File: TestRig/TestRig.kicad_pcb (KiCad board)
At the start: 2 copper layers, 62 x 48 mm, 17 parts, among them J1 USB_B_Micro, J2 AVR-ISP-6

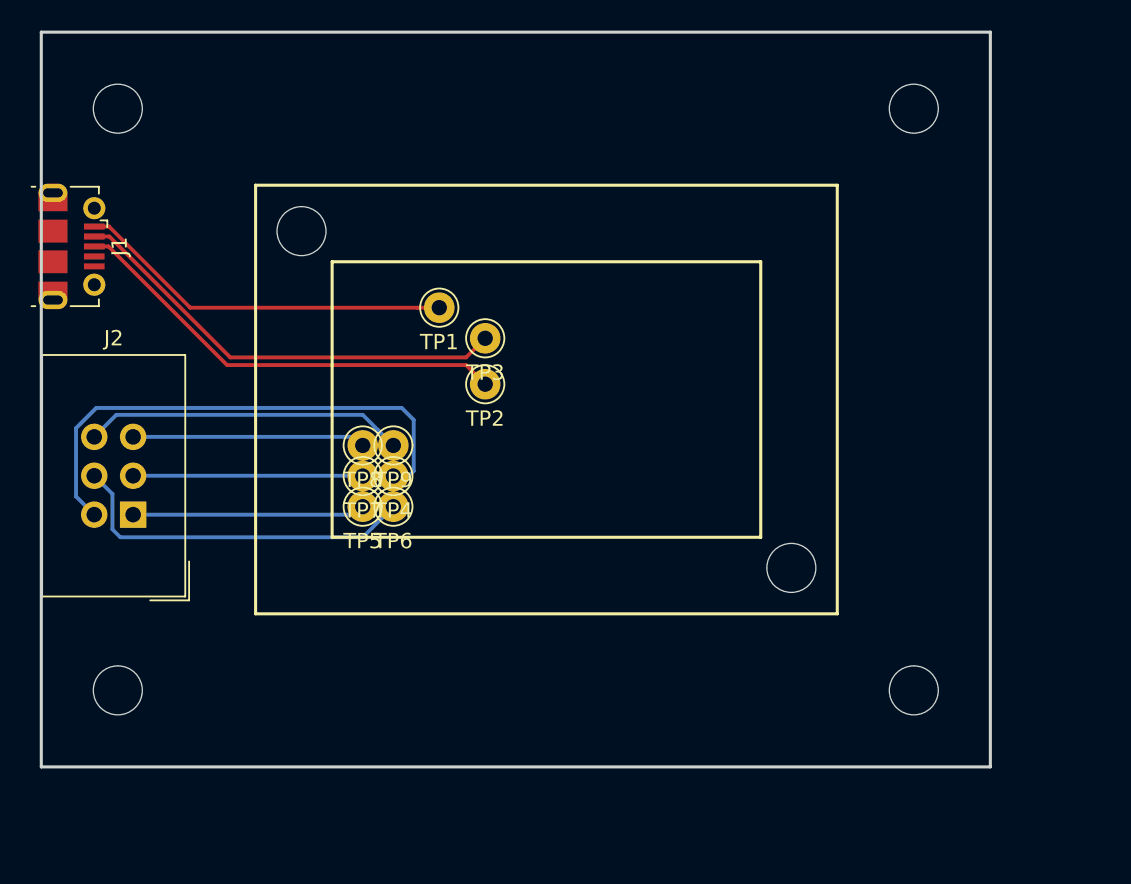
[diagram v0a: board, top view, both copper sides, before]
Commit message: Should...
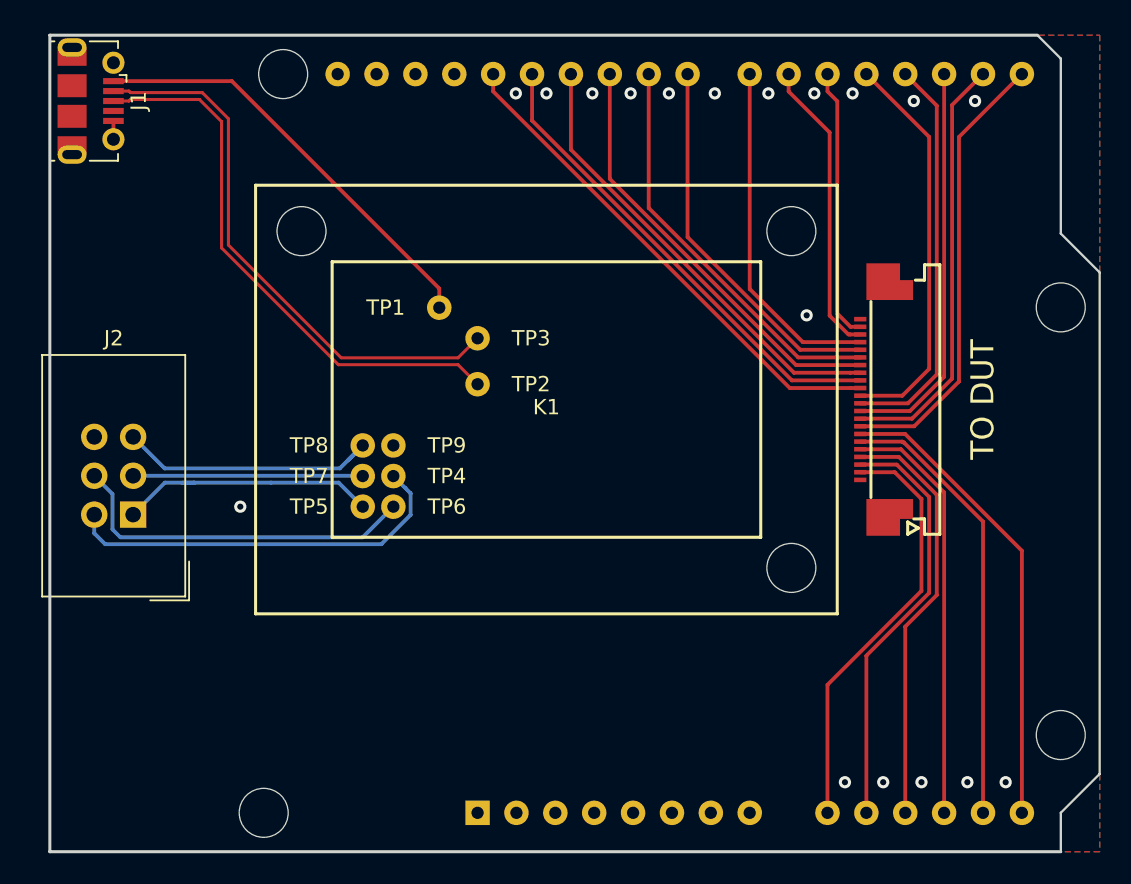
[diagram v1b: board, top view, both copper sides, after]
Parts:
- removed the MH1 at (168.0, 70.0)
- removed MH5, MH6: MountingHole, MountingHole:MountingHole_3.2mm_M3
- added A1: Arduino_UNO_R3, Module:Arduino_UNO_R3_WithMountingHoles, B.Cu at (139.5, 116.0)
- added K1: PCB Jig 3D model, TestRig:PCB_JIG, F.Cu at (144.0, 89.0)
- added K2: 3D Model Dummy, TestRig:USB_KEYBOARD_ADAPTER_V1.22_DUMMY, F.Cu at (130.0, 80.0)
- added KB1: TO DUT, RB-SMD-Connectors:FPC_0.5mm_22p-MOLEX_52437, F.Cu at (164.5, 89.0)
- TP1, TP2, TP3, TP4, TP5, TP6, TP7, TP8, TP9: footprint Connector_Pin:Pin_D1.0mm_L10.0mm -> RB-Connectors:Mill-Max_7911-0-15-20-86-14-11-0
- moved MH2 31.0 mm to (160.0, 78.0)
- moved J1 9.58 mm to (114.2, 69.5)
- moved TP2 0.50 mm to (139.5, 88.0)
- moved TP3 0.50 mm to (139.5, 85.0)
- renumbered MH4 to MH1
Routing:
- net /ROW3: track 0.00 -> 33.1 mm
- net /ROW4: track 0.00 -> 32.1 mm
- net /COL7: track 0.00 -> 30.8 mm
- net /ROW5: track 0.00 -> 29.9 mm
- net /COL3: track 0.00 -> 29.4 mm
- net /COL8: track 0.00 -> 29.2 mm
- net /COL1: track 0.00 -> 28.2 mm
- net /COL4: track 0.00 -> 27.8 mm
- net /COL9: track 0.00 -> 27.8 mm
- net /COL12: track 0.00 -> 27.7 mm
- net /COL11: track 0.00 -> 27.7 mm
- net /COL10: track 0.00 -> 27.6 mm
- net /ROW2: track 0.00 -> 26.6 mm
- net /COL6: track 0.00 -> 26.3 mm
- net /COL5: track 0.00 -> 26.2 mm
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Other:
- board size 62 x 48 mm -> 68.6 x 53.3 mm
- board text added: "PCB Test Rig for USB Keyboard Adapter v1.22 Rasmus Backman 2018"
